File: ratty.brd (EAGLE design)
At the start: 616 x 652 mm, 90 parts, among them IC2 L293DD, Q1 BS170, Q2 BS170, Q3 BS170, Q5 BS170, U1 ITG-32001:1

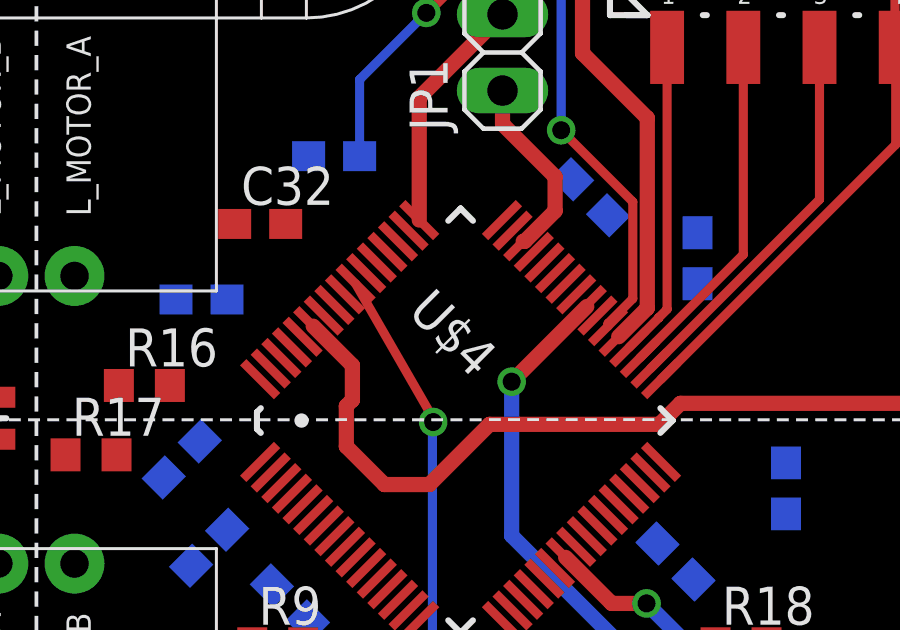
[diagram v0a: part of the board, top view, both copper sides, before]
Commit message: latest changes
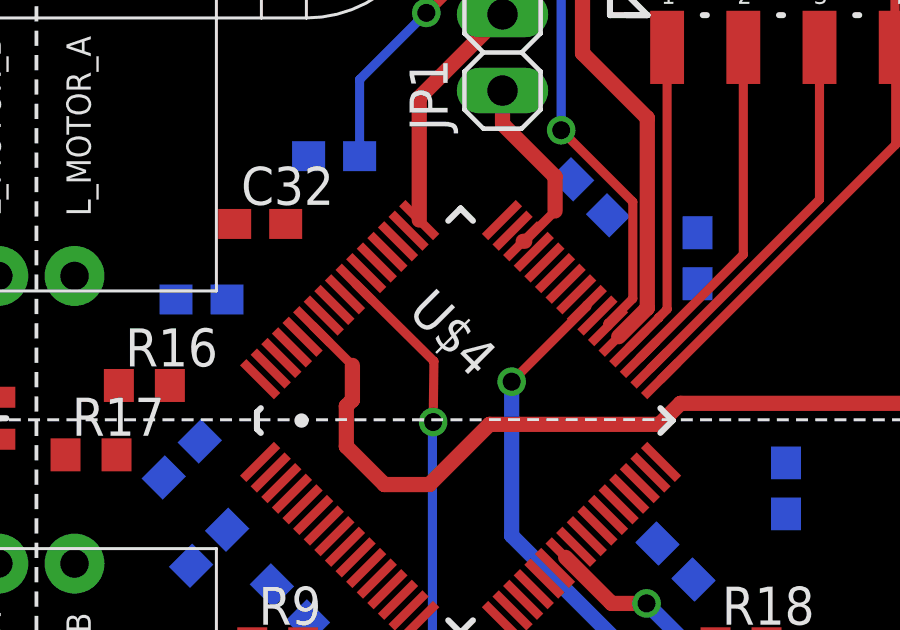
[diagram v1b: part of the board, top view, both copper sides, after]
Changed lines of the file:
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@@
 <wire x1="9.9568" y1="69.3166" x2="9.9568" y2="68.1618" width="0.508" layer="1"/>
 <wire x1="9.9568" y1="68.1618" x2="9.9178" y2="68.1228" width="0.508" layer="1"/>
-<wire x1="15.582" y1="50.3428" x2="9.9178" y2="68.1228" width="0" layer="19" extent="1-1"/>
 <wire x1="15.7852" y1="47.0408" x2="15.582" y2="50.3428" width="0" layer="19" extent="1-1"/>
 <wire x1="16.09" y1="43.9928" x2="15.7852" y2="47.0408" width="0" layer="19" extent="1-1"/>
@@
 <contactref element="U$4" pad="48"/>
 <contactref element="U$4" pad="64"/>
-<wire x1="43.442559375" y1="47.845040625" x2="48.3226" y2="76.7588" width="0" layer="19" extent="1-16"/>
+<wire x1="43.442559375" y1="47.845040625" x2="47.625" y2="44.362" width="0" layer="19" extent="16-16"/>
 <wire x1="41.10445625" y1="46.48395625" x2="43.442559375" y2="47.845040625" width="0" layer="19" extent="1-16"/>
-<wire x1="47.625" y1="44.362" x2="43.442559375" y2="47.845040625" width="0" layer="19" extent="16-16"/>
 <wire x1="46.40775625" y1="38.422940625" x2="47.625" y2="44.362" width="0" layer="19" extent="1-16"/>
+<wire x1="31.03024375" y1="39.107440625" x2="33.043440625" y2="38.422940625" width="0" layer="19" extent="1-16"/>
+<wire x1="31.94464375" y1="36.161040625" x2="33.043440625" y2="38.422940625" width="0" layer="19" extent="1-16"/>
 <wire x1="46.287359375" y1="35.703840625" x2="46.40775625" y2="38.422940625" width="0" layer="19" extent="1-16"/>
+<wire x1="30.2396" y1="43.8404" x2="32.1954" y2="46.355" width="0" layer="19" extent="1-16"/>
+<wire x1="34.6592" y1="48.6156" x2="32.1954" y2="46.355" width="0" layer="19" extent="1-16"/>
+<wire x1="34.63704375" y1="33.10475625" x2="31.94464375" y2="36.161040625" width="0" layer="19" extent="16-16"/>
+<wire x1="37.28608125" y1="34.1803" x2="34.63704375" y2="33.10475625" width="0" layer="19" extent="1-16"/>
 <wire x1="50.5714" y1="38.3912" x2="46.40775625" y2="38.422940625" width="0" layer="19" extent="1-16"/>
-<wire x1="41.8115625" y1="33.826746875" x2="46.287359375" y2="35.703840625" width="0" layer="19" extent="1-16"/>
-<wire x1="37.28608125" y1="34.1803" x2="41.8115625" y2="33.826746875" width="0" layer="19" extent="1-1"/>
-<wire x1="34.63704375" y1="33.10475625" x2="37.28608125" y2="34.1803" width="0" layer="19" extent="1-16"/>
-<wire x1="31.94464375" y1="36.161040625" x2="34.63704375" y2="33.10475625" width="0" layer="19" extent="16-16"/>
-<wire x1="33.043440625" y1="38.422940625" x2="31.94464375" y2="36.161040625" width="0" layer="19" extent="1-16"/>
-<wire x1="31.03024375" y1="39.107440625" x2="33.043440625" y2="38.422940625" width="0" layer="19" extent="1-16"/>
-<wire x1="33.043440625" y1="41.18065625" x2="33.043440625" y2="38.422940625" width="0" layer="19" extent="1-1"/>
-<wire x1="30.2396" y1="43.8404" x2="33.043440625" y2="41.18065625" width="0" layer="19" extent="1-16"/>
-<wire x1="32.1954" y1="46.355" x2="30.2396" y2="43.8404" width="0" layer="19" extent="1-16"/>
-<wire x1="34.6592" y1="48.6156" x2="32.1954" y2="46.355" width="0" layer="19" extent="1-16"/>
-<wire x1="24.2838" y1="40.578" x2="30.2396" y2="43.8404" width="0" layer="19" extent="1-16"/>
-<wire x1="44.362" y1="27.2796" x2="41.8115625" y2="33.826746875" width="0" layer="19" extent="1-1"/>
-<wire x1="62.8142" y1="38.9772" x2="50.5714" y2="38.3912" width="0" layer="19" extent="1-16"/>
+<wire x1="41.8115625" y1="33.826746875" x2="37.28608125" y2="34.1803" width="0" layer="19" extent="1-1"/>
 <wire x1="73.584096875" y1="40.3754875" x2="66.0282" y2="35.7632" width="0" layer="19" extent="1-1"/>
-<wire x1="54.825" y1="12.2682" x2="44.362" y2="27.2796" width="0" layer="19" extent="1-1"/>
-<wire x1="60.8702" y1="13.3604" x2="54.825" y2="12.2682" width="0" layer="19" extent="1-1"/>
-<wire x1="46.4684" y1="4.3434" x2="54.825" y2="12.2682" width="0" layer="19" extent="1-1"/>
-<wire x1="3.2512" y1="37.4142" x2="24.2838" y2="40.578" width="0" layer="19" extent="1-1"/>
+<wire x1="48.3226" y1="76.7588" x2="43.442559375" y2="47.845040625" width="0" layer="19" extent="1-16"/>
 </signal>
 <signal name="TO_C5_CAP">
@@
 <wire x1="35.9156" y1="40.2844" x2="36.1188" y2="40.4876" width="0.508" layer="1"/>
 <wire x1="36.1188" y1="40.4876" x2="36.1188" y2="41.64083125" width="0.508" layer="1"/>
-<wire x1="36.1188" y1="41.64083125" x2="34.81120625" y2="42.948425" width="0.508" layer="1"/>
+<wire x1="36.1188" y1="41.64083125" x2="34.81120625" y2="42.948425" width="0.3048" layer="1"/>
 </signal>
 <signal name="PB9_GYROCLK">
@@
 <wire x1="17.2974" y1="30.353" x2="17.2974" y2="31.6602" width="0.508" layer="1"/>
 <wire x1="17.2974" y1="31.6602" x2="17.2838" y2="31.6738" width="0.508" layer="1"/>
-<contactref element="C11" pad="2"/>
 <contactref element="C17" pad="2"/>
 <contactref element="C18" pad="2"/>
@@
 <contactref element="U$4" pad="63"/>
 <contactref element="U$4" pad="60"/>
+<contactref element="C11" pad="2"/>
 <wire x1="71.7444875" y1="42.6317125" x2="72.836390625" y2="43.307" width="0" layer="19" extent="1-1"/>
 <wire x1="67.7418" y1="37.3888" x2="71.7444875" y2="42.6317125" width="0" layer="19" extent="1-1"/>
@@
 <wire x1="41.1226" y1="49.6824" x2="42.8752" y2="47.9298" width="0.508" layer="1"/>
 <wire x1="42.8752" y1="47.9298" x2="42.8752" y2="46.7868" width="0.508" layer="1"/>
-<wire x1="42.8752" y1="46.7868" x2="41.86525" y2="45.77685" width="0.508" layer="1"/>
+<wire x1="42.8752" y1="46.7868" x2="41.86525" y2="45.77685" width="0.3048" layer="1"/>
 <wire x1="41.86525" y1="45.77685" x2="41.8115625" y2="45.77685" width="0.508" layer="1"/>
 </signal>
@@
 <wire x1="38.7858" y1="39.7256" x2="38.8112" y2="39.751" width="0.3048" layer="16"/>
 <via x="38.8112" y="39.751" extent="1-16" drill="0.6"/>
-<wire x1="38.8112" y1="39.751" x2="38.8112" y2="39.87185625" width="0.3048" layer="1"/>
-<wire x1="38.8112" y1="39.87185625" x2="36.22541875" y2="44.3626375" width="0.3048" layer="1"/>
+<wire x1="38.8112" y1="39.751" x2="38.8366" y2="41.77685625" width="0.3048" layer="1"/>
+<wire x1="38.8366" y1="41.77685625" x2="36.22541875" y2="44.3626375" width="0.3048" layer="1"/>
 </signal>
 <signal name="PA_7_REC_CIRCUIT_1">
@@
 <wire x1="41.4274" y1="35.9664" x2="41.4274" y2="41.0972" width="0.508" layer="16"/>
 <via x="41.4274" y="41.0972" extent="1-16" drill="0.6"/>
-<wire x1="41.4274" y1="41.0972" x2="43.932884375" y2="43.602684375" width="0.508" layer="1"/>
+<wire x1="41.4274" y1="41.0972" x2="43.932884375" y2="43.602684375" width="0.3048" layer="1"/>
 <wire x1="43.932884375" y1="43.602684375" x2="43.932884375" y2="43.65553125" width="0.3048" layer="1"/>
 <wire x1="43.932884375" y1="43.65553125" x2="72.771" y2="54.825" width="0" layer="19" extent="1-1"/>
